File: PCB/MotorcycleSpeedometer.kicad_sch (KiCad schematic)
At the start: 20 parts, among them J1 Conn_01x08, J2 Conn_01x06, J3 Conn_01x10, J4 Conn_01x08, J5 Conn_02x08_Top_Bottom, Q1 2N7002, Q2 2N7002, Q3 2N7002, Q4 2N7002, Q5 2N7002

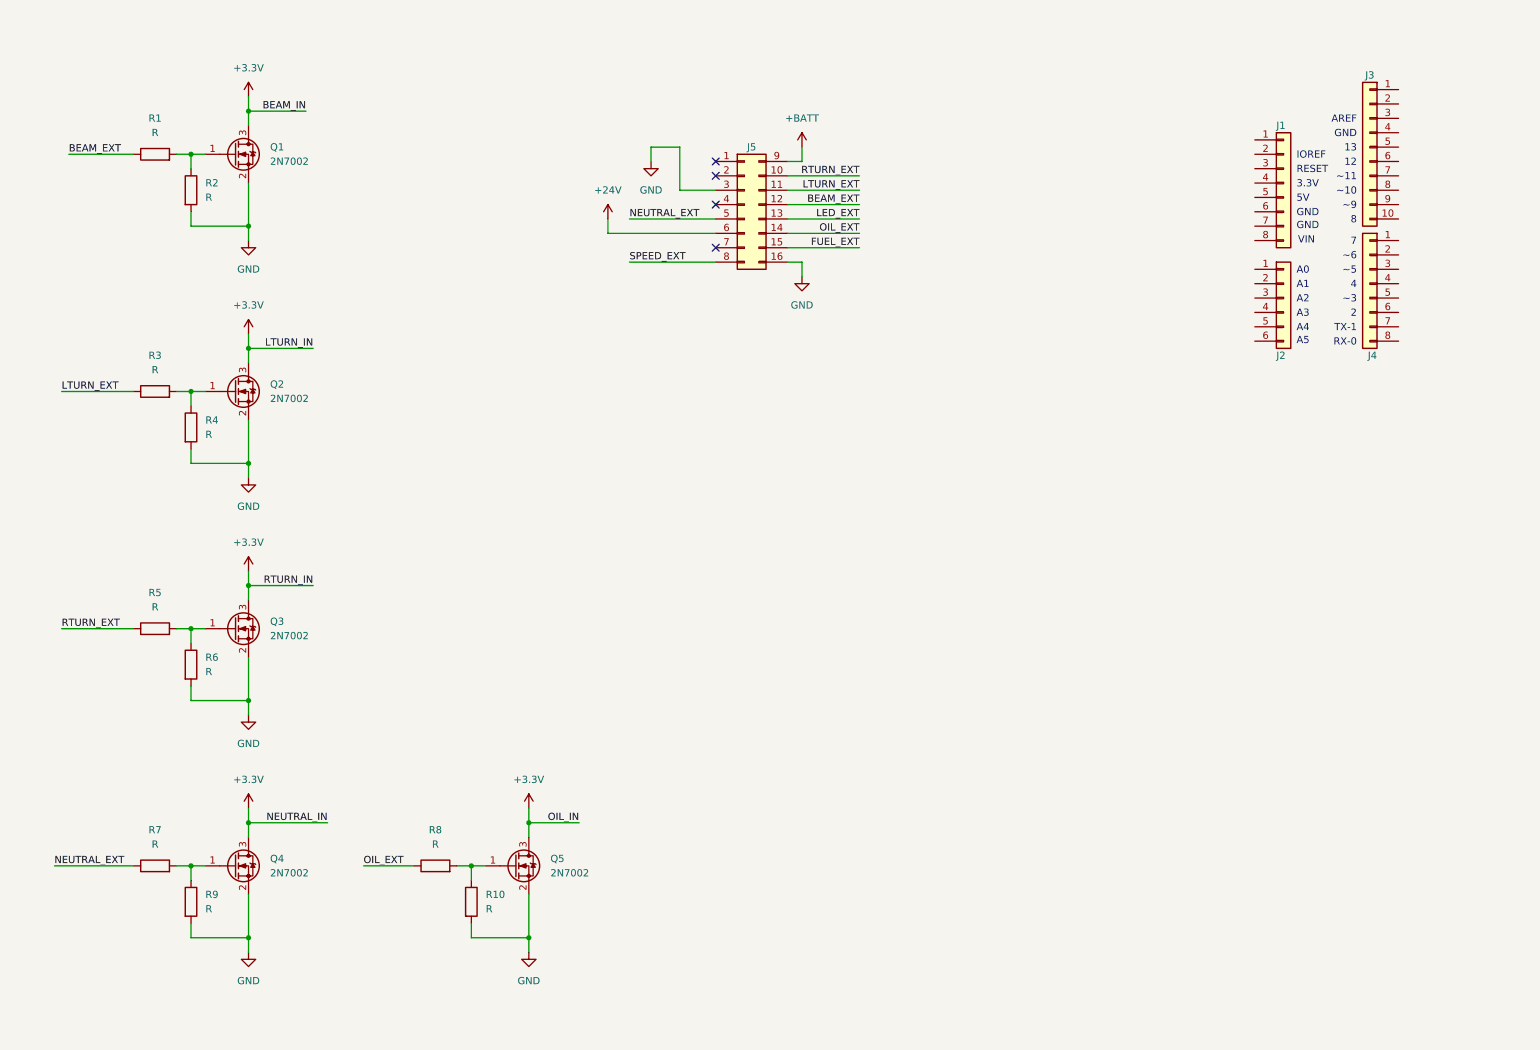
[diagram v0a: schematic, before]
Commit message: Updated PCB
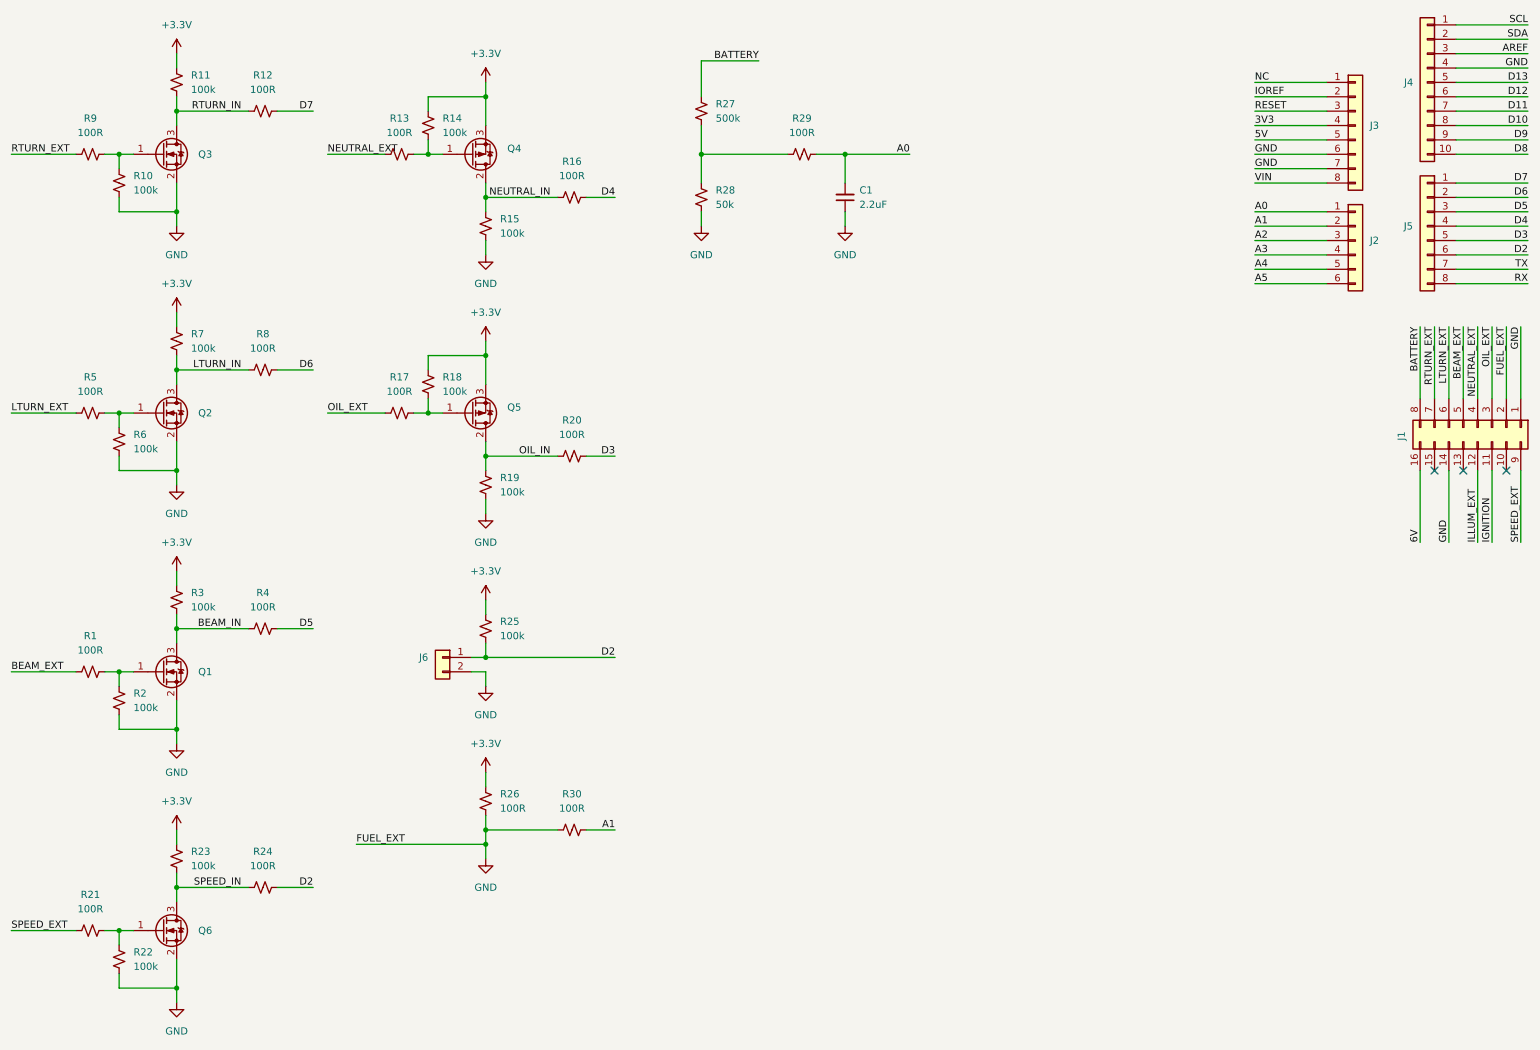
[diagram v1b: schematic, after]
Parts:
- removed J1, J4: Conn_01x08, symbol Connector_Generic:Conn_01x08
- removed J3: Conn_01x10, symbol Connector_Generic:Conn_01x10
- removed J5: Conn_02x08_Top_Bottom, symbol Connector_Generic:Conn_02x08_Top_Bottom
- removed Q4, Q5: 2N7002, Package_TO_SOT_SMD:SOT-23, symbol Transistor_FET:2N7002
- removed R10, R2, R3, R4, R5, R6, R7, R8, R9: R, symbol Device:R
- added C1: 2.2uF, symbol Device:C_Small
- added J1: Conn_02x08_Odd_Even, Connector_PinHeader_2.54mm:PinHeader_2x08_P2.54mm_Vertical, symbol Connector_Generic:Conn_02x08_Top_Bottom
- added J3, J5: Conn_01x08, symbol Connector_Generic:Conn_01x08
- added J4: Conn_01x10, symbol Connector_Generic:Conn_01x10
- added J6: Conn_01x02, symbol Connector_Generic:Conn_01x02
- added Q4, Q5: Q_PMOS_GDS, symbol Device:Q_PMOS_GDS
- added Q6: 2N7002, Package_TO_SOT_SMD:SOT-23, symbol Transistor_FET:2N7002
- added R10, R11, R14, R15, R18, R19, R2, R22, R23, R25, R3, R6, R7: 100k, Resistor_SMD:R_0603_1608Metric, symbol Device:R_Small_US
- added R12, R13, R16, R17, R20, R21, R24, R26, R29, R30, R4, R5, R8, R9: 100R, Resistor_SMD:R_0603_1608Metric, symbol Device:R_Small_US
- added R27: 500k, Resistor_SMD:R_0603_1608Metric, symbol Device:R_Small_US
- added R28: 50k, Resistor_SMD:R_0603_1608Metric, symbol Device:R_Small_US
- R1: value R -> 100R; footprint (none) -> Resistor_SMD:R_0603_1608Metric; symbol Device:R -> Device:R_Small_US
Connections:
- net +3.3V: now also Q4.3 (S), Q5.3 (S), R11.2, R14.2, R18.2, R23.2, R25.2, R26.2, R3.2, R7.2; no longer Q1.3 (D), Q2.3 (D), Q3.3 (D)
- net BEAM_EXT: now also J1.5 (Pin_5)
- net GND: now also C1.1, J1.1 (Pin_1), J1.14 (Pin_14), J1.2 (Pin_2), J3.6 (Pin_6), J3.7 (Pin_7), J4.4 (Pin_4), J6.2 (Pin_2), Q6.2 (S), R10.1, R15.1, R19.1, R2.1, R22.1, R26.1, R28.1, R30.1, R6.1
- net LTURN_EXT: now also J1.6 (Pin_6), R5.1
- net NEUTRAL_EXT: now also J1.4 (Pin_4), R13.1
- net OIL_EXT: now also J1.3 (Pin_3), R17.1
- net RTURN_EXT: now also J1.7 (Pin_7), R9.1
- net SPEED_EXT: now also J1.9 (Pin_9), R21.1
- net at Q3.1 (G): now also R10.2, R9.2
- net at Q2.1 (G): now also R5.2, R6.2
- net A0: now reaches J2.1 (Pin_1)
- net A0: now also C1.2, R29.2
- net A1: now reaches J2.2 (Pin_2)
- net A1: now also R30.2
- net A2: now reaches J2.3 (Pin_3)
- net A3: now reaches J2.4 (Pin_4)
- net A4: now reaches J2.5 (Pin_5)
- net A5: now reaches J2.6 (Pin_6)
- net at Q1.1 (G), R1.2: now also R2.2
- new net: Q6.1 (G), R21.2, R22.2
- new net: R27.1, R28.2, R29.1
- new net: Q4.1 (G), R13.2, R14.1
- new net: Q5.1 (G), R17.2, R18.1
- new net 3V3: J3.4 (Pin_4)
- new net 5V: J3.5 (Pin_5)
- new net 6V: J1.16 (Pin_16)
- new net AREF: J4.3 (Pin_3)
- new net BATTERY: J1.8 (Pin_8), R27.2
- new net BEAM_IN: Q1.3 (D), R3.1, R4.1
- new net D10: J4.8 (Pin_8)
- new net D11: J4.7 (Pin_7)
- new net D12: J4.6 (Pin_6)
- new net D13: J4.5 (Pin_5)
- new net D2: J5.6 (Pin_6), J6.1 (Pin_1), R24.2, R25.1
- new net D3: J5.5 (Pin_5), R20.2
- new net D4: J5.4 (Pin_4), R16.2
- new net D5: J5.3 (Pin_3), R4.2
- new net D6: J5.2 (Pin_2), R8.2
- new net D7: J5.1 (Pin_1), R12.2
- new net D8: J4.10 (Pin_10)
- new net D9: J4.9 (Pin_9)
- new net IGNITION: J1.11 (Pin_11)
- new net ILLUM_EXT: J1.12 (Pin_12)
- new net IOREF: J3.2 (Pin_2)
- new net LTURN_IN: Q2.3 (D), R7.1, R8.1
- new net NC: J3.1 (Pin_1)
- new net NEUTRAL_IN: Q4.2 (D), R15.2, R16.1
- new net OIL_IN: Q5.2 (D), R19.2, R20.1
- new net RESET: J3.3 (Pin_3)
- new net RTURN_IN: Q3.3 (D), R11.1, R12.1
- new net RX: J5.8 (Pin_8)
- new net SCL: J4.1 (Pin_1)
- new net SDA: J4.2 (Pin_2)
- new net SPEED_IN: Q6.3 (D), R23.1, R24.1
- new net TX: J5.7 (Pin_7)
- new net VIN: J3.8 (Pin_8)
- no-connect marks 4 -> 3
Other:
- note removed: "12"
- note removed: "13"
- note removed: "2"
- note removed: "3.3V"
- note removed: "4"
- note removed: "5V"
- note removed: "7"
- note removed: "8"
- note removed: "A0"
- note removed: "A1"
- note removed: "A2"
- note removed: "A3"
- note removed: "A4"
- note removed: "A5"
- note removed: "AREF"
- note removed: "GND"
- note removed: "IOREF"
- note removed: "RESET"
- note removed: "RX-0"
- note removed: "TX-1"
- note removed: "VIN"
- note removed: "~10"
- note removed: "~11"
- note removed: "~3"
- note removed: "~5"
- note removed: "~6"
- note removed: "~9"
- moved on the sheet: Q1
